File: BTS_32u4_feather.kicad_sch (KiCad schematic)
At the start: 28 parts, among them J1 USB4105-GF-A, J2 Conn_01x04, J6 Analog, J7 Digital, U1 ATmega32U4-A, U3 AMS1117-3.3, Y1 8Mhz Crystal

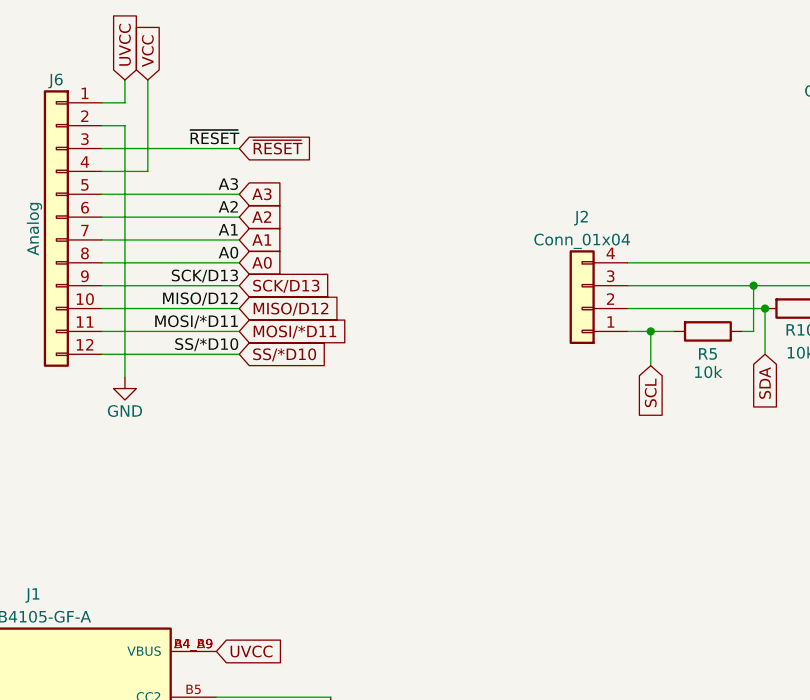
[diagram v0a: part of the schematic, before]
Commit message: wip
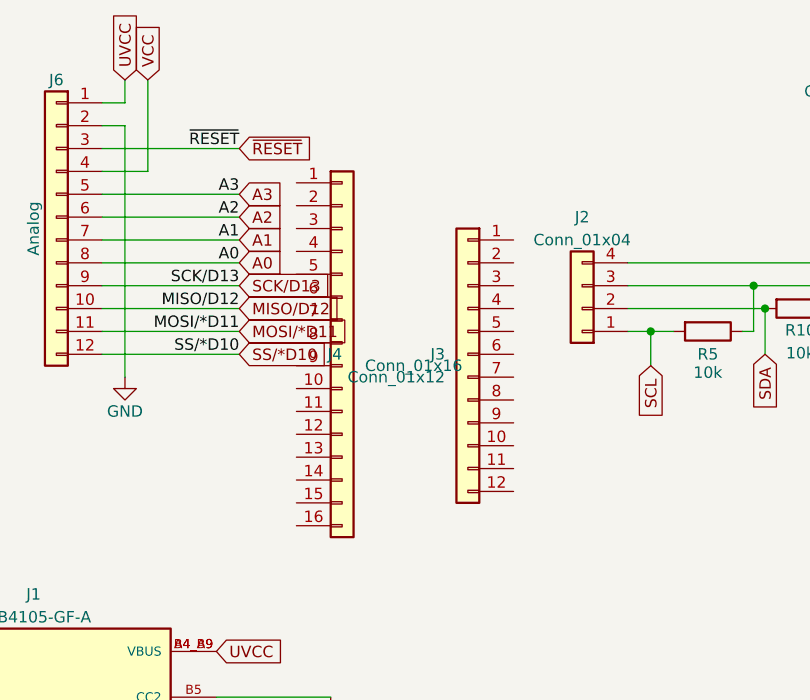
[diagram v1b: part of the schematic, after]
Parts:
- added J3: Conn_01x12, symbol Connector_Generic:Conn_01x12
- added J4: Conn_01x16, symbol Connector_Generic:Conn_01x16
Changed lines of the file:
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@@
+	)
+	(symbol
+		(lib_id "Connector_Generic:Conn_01x12")
+		(at 109.22 104.14 0)
+		(mirror y)
+		(unit 1)
+		(exclude_from_sim no)
+		(in_bom yes)
+		(on_board yes)
+		(dnp no)
+		(property "Reference" "J3"
+			(at 106.68 104.1399 0)
+			(effects
+				(font
+					(size 1.27 1.27)
+				)
+				(justify left)
+			)
+		)
+		(property "Value" "Conn_01x12"
+			(at 106.68 106.6799 0)
+			(effects
+				(font
+					(size 1.27 1.27)
+				)
+				(justify left)
+			)
+		)
+		(property "Footprint" ""
+			(at 109.22 104.14 0)
+			(effects
+				(font
+					(size 1.27 1.27)
+				)
+				(hide yes)
+			)
+		)
+		(property "Datasheet" "~"
+			(at 109.22 104.14 0)
+			(effects
+				(font
+					(size 1.27 1.27)
+				)
+				(hide yes)
+			)
+		)
+		(property "Description" "Generic connector, single row, 01x12, script generated (kicad-library-utils/schlib/autogen/connector/)"
+			(at 109.22 104.14 0)
+			(effects
+				(font
+					(size 1.27 1.27)
+				)
+				(hide yes)
+			)
+		)
+		(pin "6"
+		)
+		(pin "10"
+		)
+		(pin "7"
+		)
+		(pin "1"
+		)
+		(pin "12"
+		)
+		(pin "8"
+		)
+		(pin "5"
+		)
+		(pin "9"
+		)
+		(pin "3"
+		)
+		(pin "2"
+		)
+		(pin "11"
+		)
+		(pin "4"
+		)
+		(instances
+			(project ""
+				(path "/e63e39d7-6ac0-4ffd-8aa3-1841a4541b55"
+					(reference "J3")
+					(unit 1)
+				)
+			)
+		)
+	)
+	(symbol
+		(lib_id "Connector_Generic:Conn_01x16")
+		(at 95.25 102.87 0)
+		(unit 1)
+		(exclude_from_sim no)
+		(in_bom yes)
+		(on_board yes)
+		(dnp no)
+		(property "Reference" "J4"
+			(at 95.25 104.1399 0)
+			(effects
+				(font
+					(size 1.27 1.27)
+				)
+				(justify right)
+			)
+		)
+		(property "Value" "Conn_01x16"
+			(at 97.79 105.4099 0)
+			(effects
+				(font
+					(size 1.27 1.27)
+				)
+				(justify left)
+			)
+		)
+		(property "Footprint" ""
+			(at 95.25 102.87 0)
+			(effects
+				(font
+					(size 1.27 1.27)
+				)
+				(hide yes)
+			)
+		)
+		(property "Datasheet" "~"
+			(at 95.25 102.87 0)
+			(effects
+				(font
+					(size 1.27 1.27)
+				)
+				(hide yes)
+			)
+		)
+		(property "Description" "Generic connector, single row, 01x16, script generated (kicad-library-utils/schlib/autogen/connector/)"
+			(at 95.25 102.87 0)
+			(effects
+				(font
+					(size 1.27 1.27)
+				)
+				(hide yes)
+			)
+		)
+		(pin "6"
+		)
+		(pin "12"
+		)
+		(pin "16"
+		)
+		(pin "4"
+		)
+		(pin "5"
+		)
+		(pin "2"
+		)
+		(pin "13"
+		)
+		(pin "3"
+		)
+		(pin "7"
+		)
+		(pin "9"
+		)
+		(pin "10"
+		)
+		(pin "1"
+		)
+		(pin "15"
+		)
+		(pin "11"
+		)
+		(pin "14"
+		)
+		(pin "8"
+		)
+		(instances
+			(project ""
+				(path "/e63e39d7-6ac0-4ffd-8aa3-1841a4541b55"
+					(reference "J4")
+					(unit 1)
+				)
+			)
+		)
 	)
 	(symbol
